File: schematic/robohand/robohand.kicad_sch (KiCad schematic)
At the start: 3 parts, among them M1 Motor_Servo, U1 ESP32-CAM

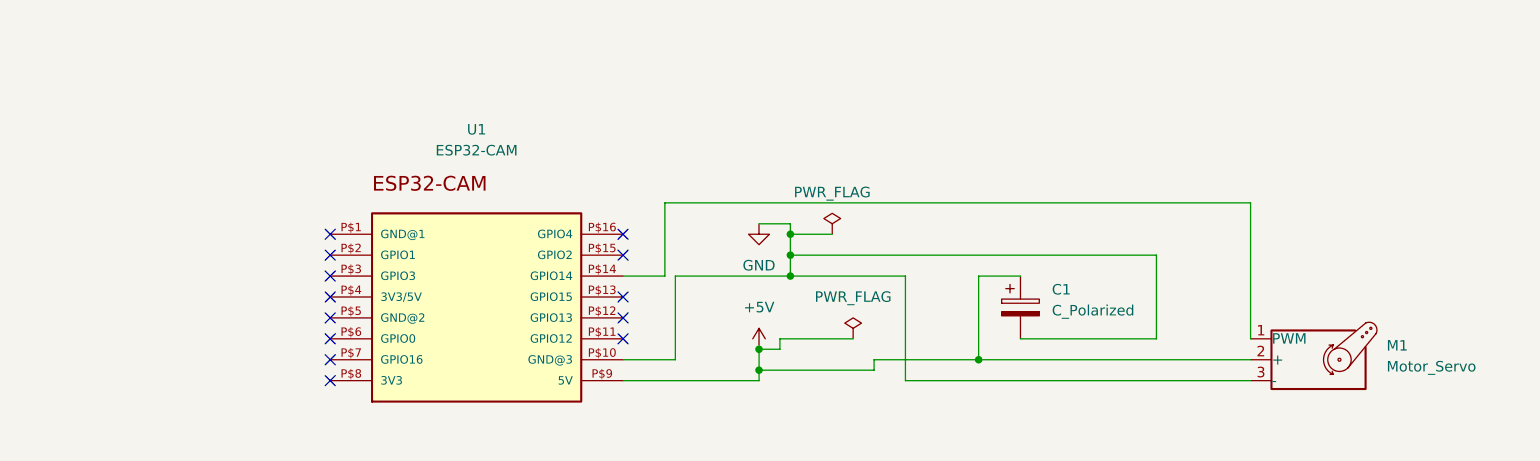
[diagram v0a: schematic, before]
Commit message: full CAD hand done
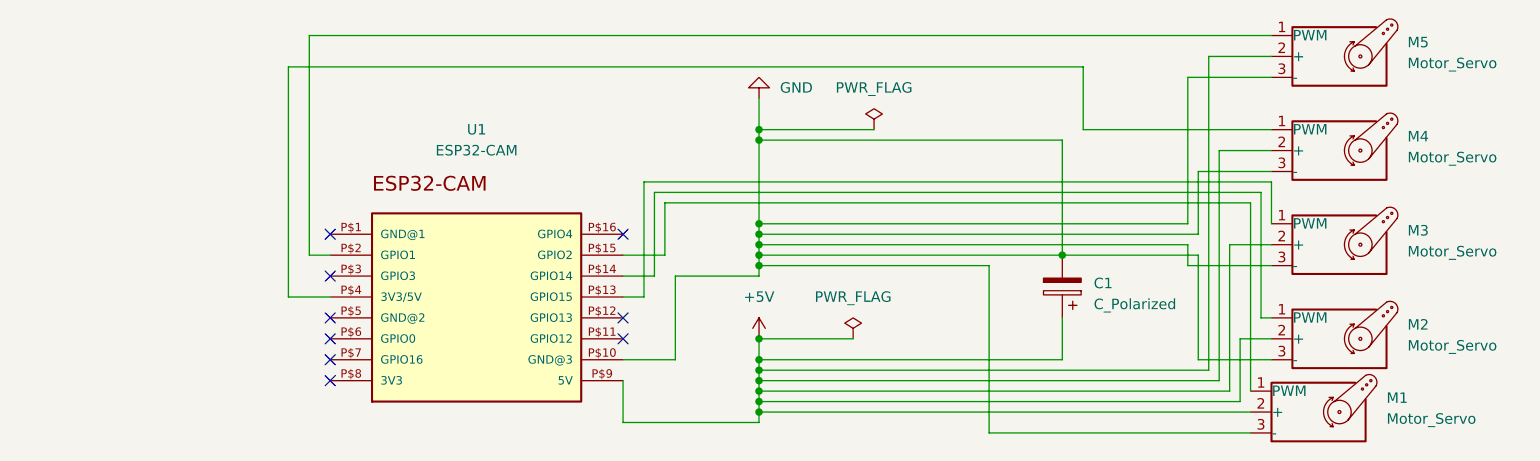
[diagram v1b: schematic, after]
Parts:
- added M2, M3, M4, M5: Motor_Servo, symbol Motor:Motor_Servo
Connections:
- net +5V: now also M2.2 (+), M3.2 (+), M4.2 (+), M5.2 (+)
- net GND: now also M2.3 (-), M3.3 (-), M4.3 (-), M5.3 (-)
- net at U1.P$13 (GPIO15): now also M3.1 (PWM)
- net at U1.P$14 (GPIO14): now also M2.1 (PWM); no longer M1.1 (PWM)
- net at U1.P$15 (GPIO2): now also M1.1 (PWM)
- net at U1.P$2 (GPIO1): now also M5.1 (PWM)
- net at U1.P$4 (3V3/5V): now also M4.1 (PWM)
- no-connect marks 13 -> 9
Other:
- moved on the sheet: C1, M1

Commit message: july 2nd
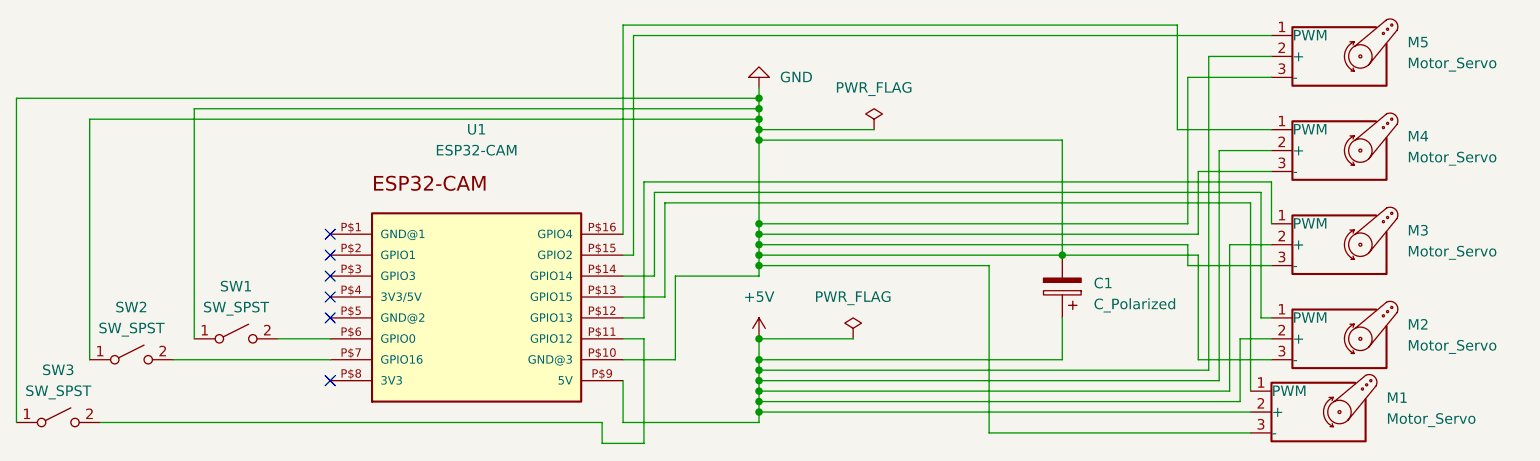
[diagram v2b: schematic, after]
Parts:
- added SW1, SW2, SW3: SW_SPST, Button_Switch_THT:SW_PUSH_6mm_H5mm, symbol Switch:SW_SPST
- C1: footprint (none) -> Capacitor_THT:CP_Radial_D5.0mm_P2.50mm
- M1, M2, M3, M4, M5: footprint (none) -> Connector_PinHeader_2.54mm:PinHeader_1x03_P2.54mm_Vertical
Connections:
- net GND: now also SW1.1 (A), SW2.1 (A), SW3.1 (A)
- net at U1.P$11 (GPIO12): now also SW3.2 (B)
- net at U1.P$12 (GPIO13): now also M3.1 (PWM)
- net at U1.P$13 (GPIO15): now also M1.1 (PWM); no longer M3.1 (PWM)
- net at U1.P$15 (GPIO2): now also M5.1 (PWM); no longer M1.1 (PWM)
- net at U1.P$16 (GPIO4): now also M4.1 (PWM)
- net at U1.P$2 (GPIO1): no longer M5.1 (PWM)
- net at U1.P$4 (3V3/5V): no longer M4.1 (PWM)
- net at U1.P$6 (GPIO0): now also SW1.2 (B)
- net at U1.P$7 (GPIO16): now also SW2.2 (B)
- no-connect marks 9 -> 6
